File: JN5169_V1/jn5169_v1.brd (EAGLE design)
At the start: 29 x 16.1 mm, 30 parts, among them Y1 32MHZ

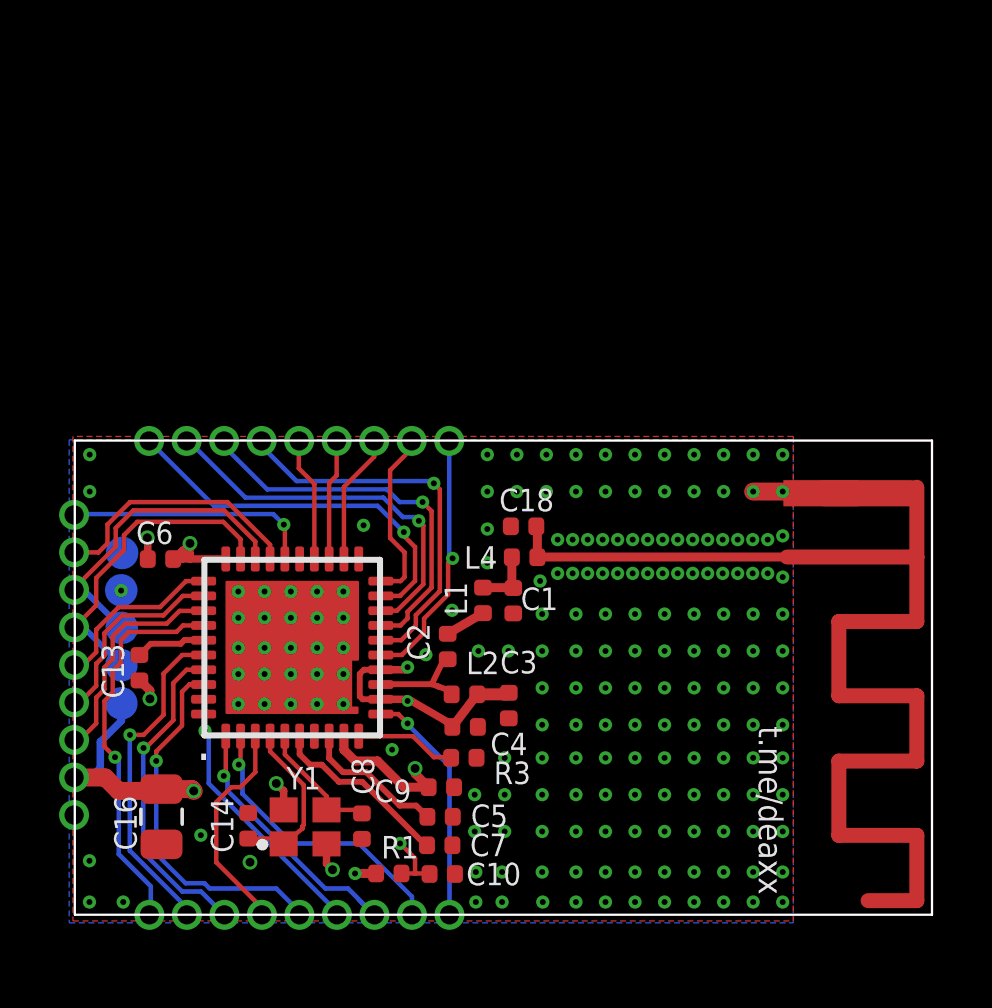
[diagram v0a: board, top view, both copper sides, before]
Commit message: Add files via upload
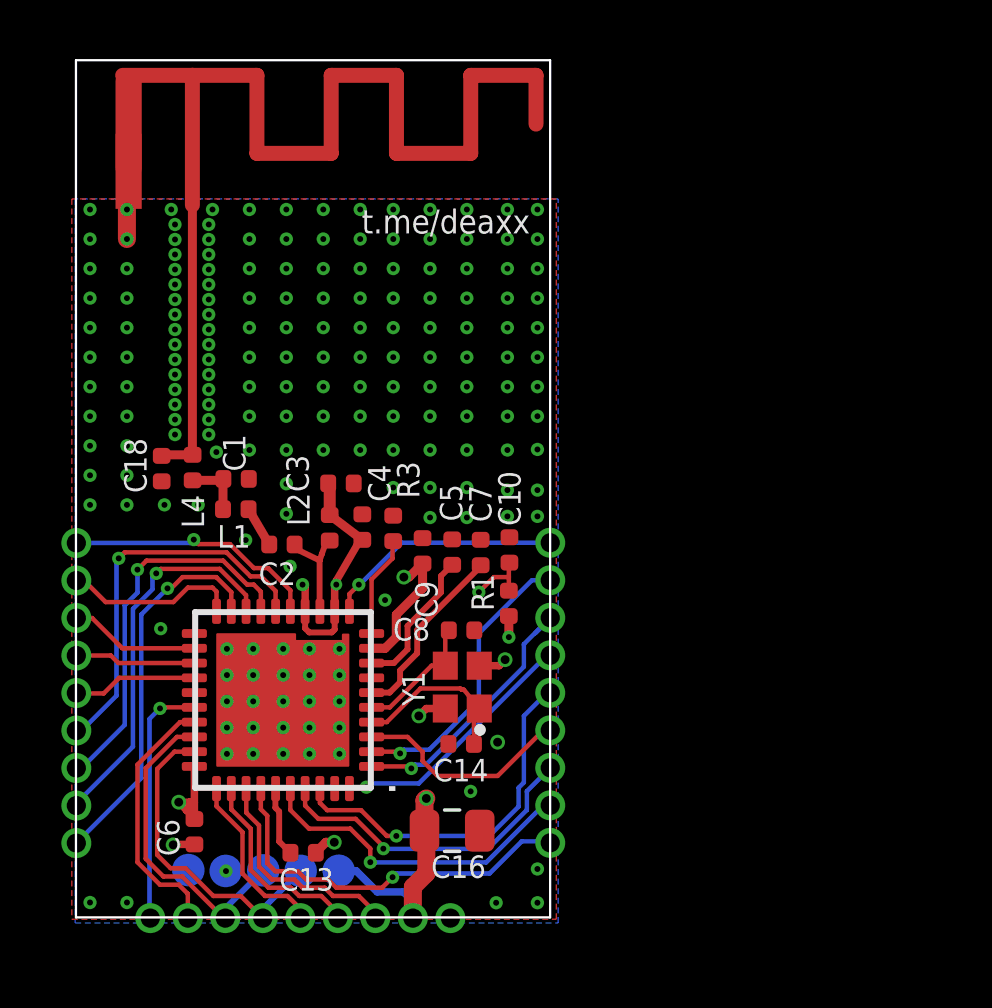
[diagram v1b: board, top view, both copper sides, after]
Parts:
- moved E1 24.3 mm to (1.99, 24.2), turned to 270 degrees
- moved J2 13.9 mm to (2.72, 0.01), turned to 0 degrees
- moved J1 13.1 mm to (0.22, 12.7), turned to 270 degrees
- moved J3 13.1 mm to (16.3, 12.7), turned to 270 degrees
- moved C18 12.4 mm to (3.11, 15.2), turned to 270 degrees
- moved L4 11.6 mm to (4.15, 15.3), turned to 270 degrees
- moved C10 11.2 mm to (14.9, 12.5), turned to 270 degrees
- moved GND 11.0 mm to (4.01, 1.64), turned to 270 degrees
- moved C1 10.2 mm to (5.62, 14.9), turned to 180 degrees
- moved TDO 10.1 mm to (5.27, 1.61), turned to 270 degrees
- moved C7 10.0 mm to (13.9, 12.4), turned to 270 degrees
- moved R1 10.0 mm to (14.9, 10.7), turned to 90 degrees
- moved C16 9.85 mm to (12.9, 2.97), turned to 0 degrees
- moved TX 9.50 mm to (6.54, 1.63), turned to 270 degrees
- moved C3 9.43 mm to (9.17, 14.7), turned to 180 degrees
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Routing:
- net SPIMISO: track 15.7 -> 16.5 mm
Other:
- board size 29 x 16.1 mm -> 16.1 x 29 mm
